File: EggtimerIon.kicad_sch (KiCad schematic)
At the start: 33 parts, among them J1 Conn_01x02, J2 Conn_01x03, J3 B2B-PH-K-S, Q1 IRLML6244, Q2 IRLML6244, U1 ESP32-WROOM-32-N4, U2 MPU-6050, U3 MS5611-01BA, U5 AP2112K-3.3

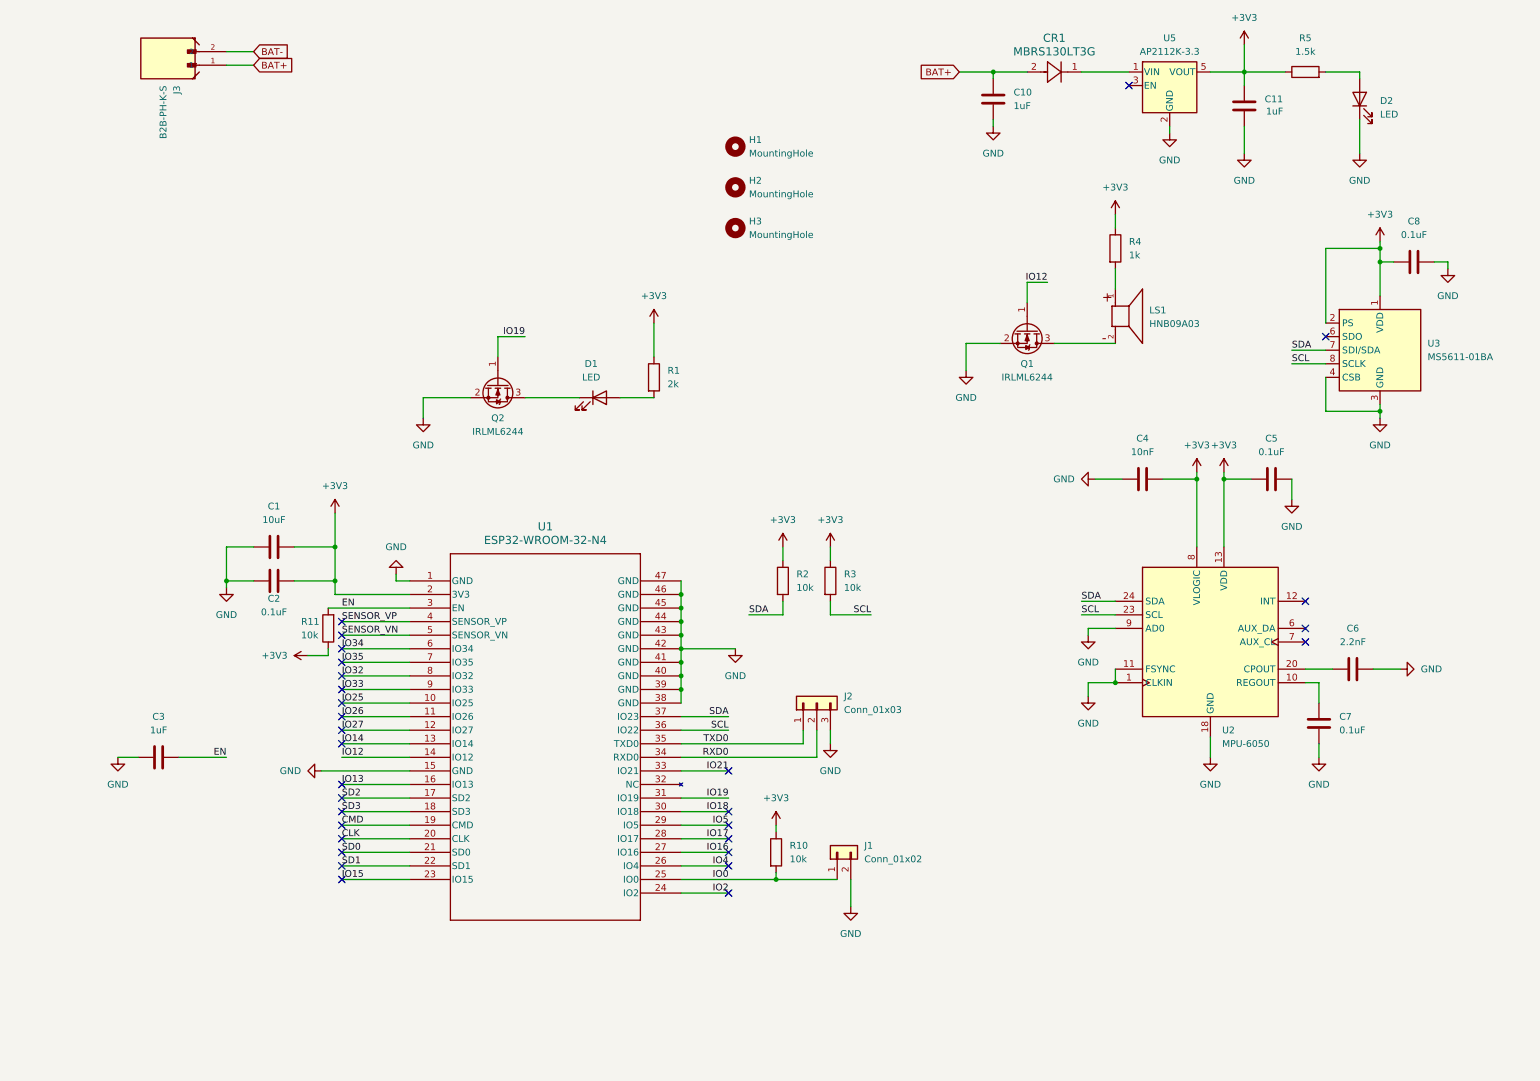
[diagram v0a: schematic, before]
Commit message: work
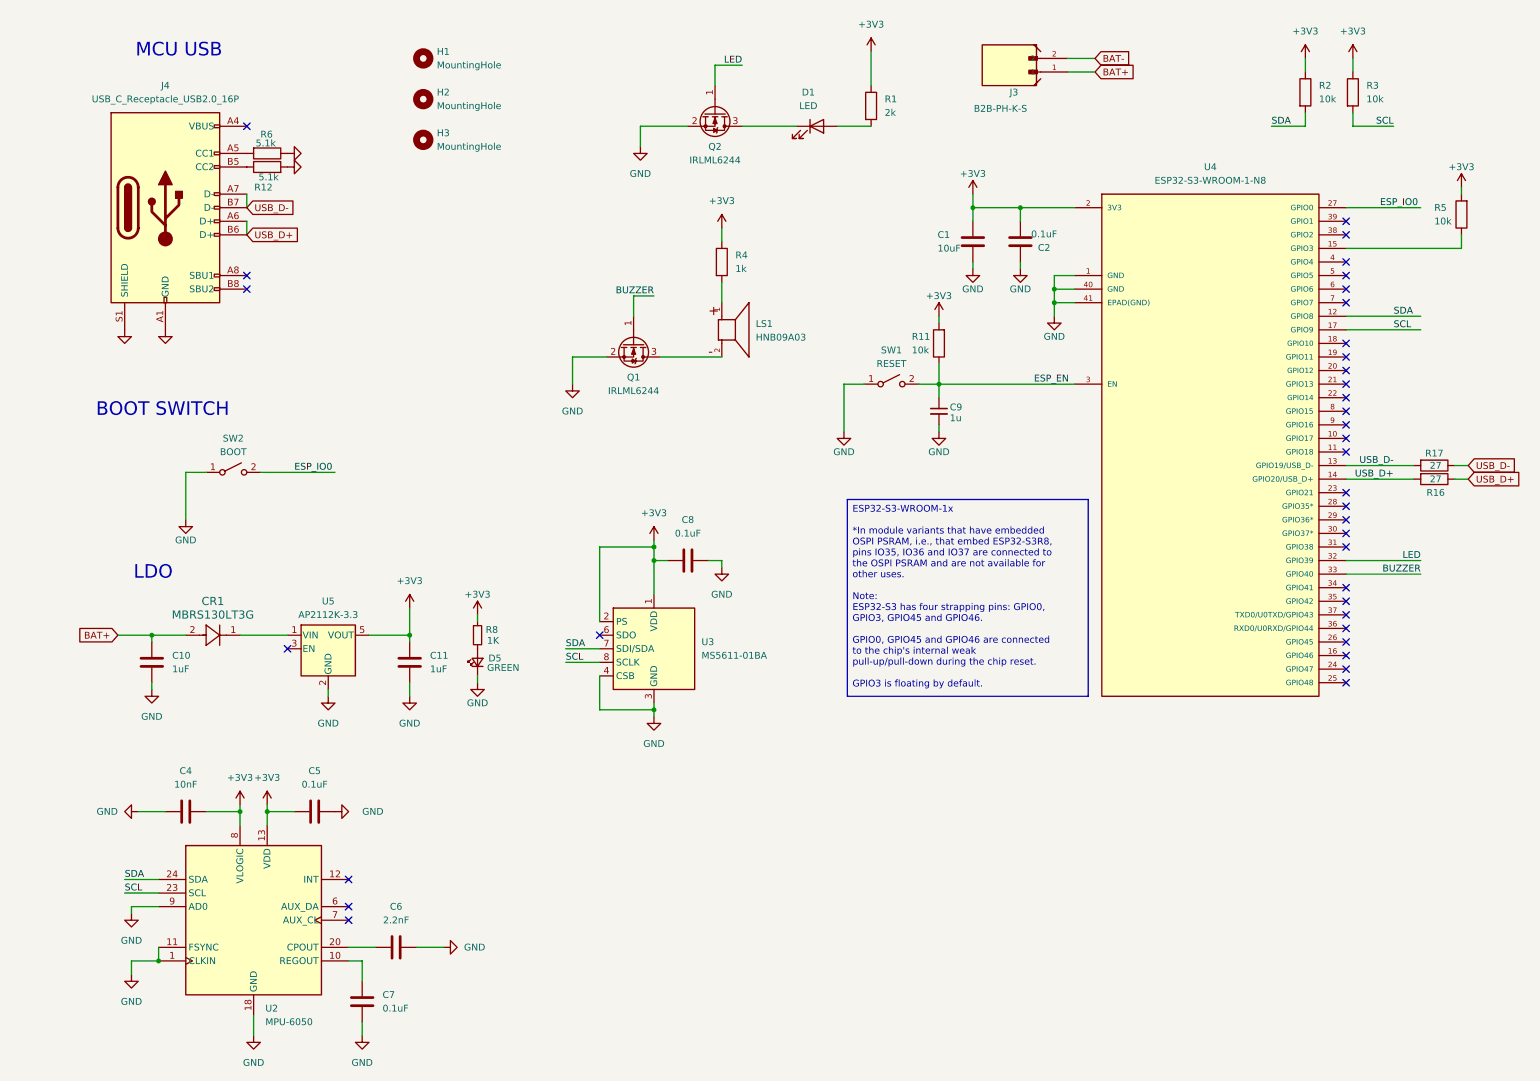
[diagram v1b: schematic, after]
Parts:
- removed C3: 1uF, Capacitor_SMD:C_0402_1005Metric, symbol Device:C
- removed D2: LED, LED_SMD:LED_0603_1608Metric, symbol Device:LED
- removed J1: Conn_01x02, Connector_PinHeader_2.54mm:PinHeader_1x02_P2.54mm_Vertical, symbol Connector_Generic:Conn_01x02
- removed J2: Conn_01x03, Connector_PinHeader_2.54mm:PinHeader_1x03_P2.54mm_Vertical, symbol Connector_Generic:Conn_01x03
- removed R10: 10k, Capacitor_SMD:C_0402_1005Metric, symbol Device:R
- removed U1: ESP32-WROOM-32-N4, RF_Module:ESP32-WROOM-32, symbol ESP32-WROOM-32-N4:ESP32-WROOM-32-N4
- added C9: 1u, Capacitor_SMD:C_0603_1608Metric, symbol Morten_Library.kicad_sym_9:C_Small
- added D5: GREEN, LED_SMD:LED_0603_1608Metric, symbol Morten_Library.kicad_sym_9:LED_Small
- added J4: USB_C_Receptacle_USB2.0_16P, Connector_USB:USB_C_Receptacle_Palconn_UTC16-G, symbol Connector:USB_C_Receptacle_USB2.0_16P
- added R12, R6: 5.1k, Resistor_SMD:R_0402_1005Metric, symbol Device:R
- added R16, R17: 27, Resistor_SMD:R_0402_1005Metric, symbol Device:R
- added R8: 1K, Resistor_SMD:R_0402_1005Metric, symbol Morten_Library.kicad_sym_9:R_Small
- added SW1: RESET, Button_Switch_SMD:SW_SPST_B3U-1000P, symbol Morten_Library.kicad_sym_9:SW_SPST
- added SW2: BOOT, Button_Switch_SMD:SW_SPST_B3U-1000P, symbol Morten_Library.kicad_sym_9:SW_SPST
- added U4: ESP32-S3-WROOM-1-N8, RF_Module:ESP32-S3-WROOM-1, symbol Morten_Library.kicad_sym_9:ESP32-S3-WROOM-1x-N8R8
- R5: value 1.5k -> 10k; LCSC C25867 -> C25744
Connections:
- net EN is gone; now on net +3V3: R11.2
- net +3V3: now also R5.2, R8.1, U4.2 (3V3); no longer R11.1, R5.1
- net GND: now also C9.2, D5.1 (K), J4.A1 (GND), J4.A12 (GND), J4.B1 (GND), J4.B12 (GND), J4.S1 (SHIELD), R12.2, R6.1, SW1.1 (A), SW2.1 (A), U4.1 (GND), U4.40 (GND), U4.41 (EPAD(GND))
- net SCL: now also U4.17 (GPIO9)
- net SDA: now also U4.12 (GPIO8)
- net IO12 renamed BUZZER
- net BUZZER: now also U4.33 (GPIO40)
- net IO19 renamed LED
- net LED: now also U4.32 (GPIO39)
- new net: J4.A4 (VBUS), J4.A9 (VBUS), J4.B4 (VBUS), J4.B9 (VBUS)
- new net: J4.A5 (CC1), R6.2
- new net: J4.B5 (CC2), R12.1
- new net: D5.2 (A), R8.2
- new net: R5.1, U4.15 (GPIO3)
- new net ESP_EN: C9.1, R11.1, SW1.2 (B), U4.3 (EN)
- new net ESP_IO0: SW2.2 (B), U4.27 (GPIO0)
- new net USB_D+: J4.A6 (D+), J4.B6 (D+), R16.1, R16.2, U4.14 (GPIO20/USB_D+)
- new net USB_D-: J4.A7 (D-), J4.B7 (D-), R17.1, R17.2, U4.13 (GPIO19/USB_D-)
- no-connect marks 30 -> 36
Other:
- note added: "BOOT SWITCH"
- note added: "LDO"
- note added: "MCU USB"
- moved on the sheet: C1, C10, C11, C2, C4, C5, C6, C7, C8, CR1, D1, H1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

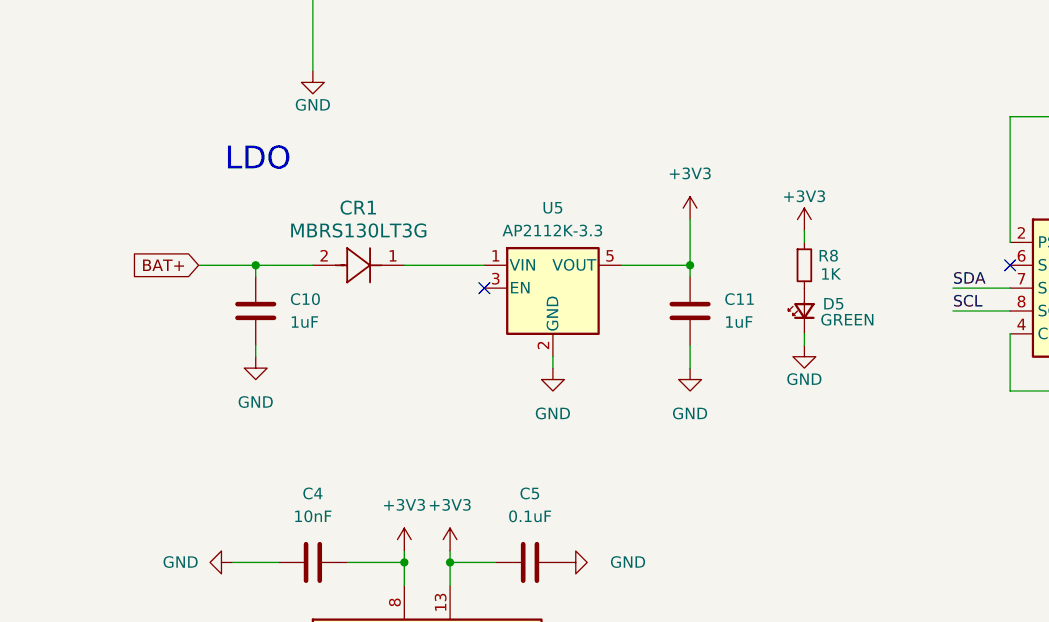
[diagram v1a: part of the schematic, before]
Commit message: Updates
work towards S3 module
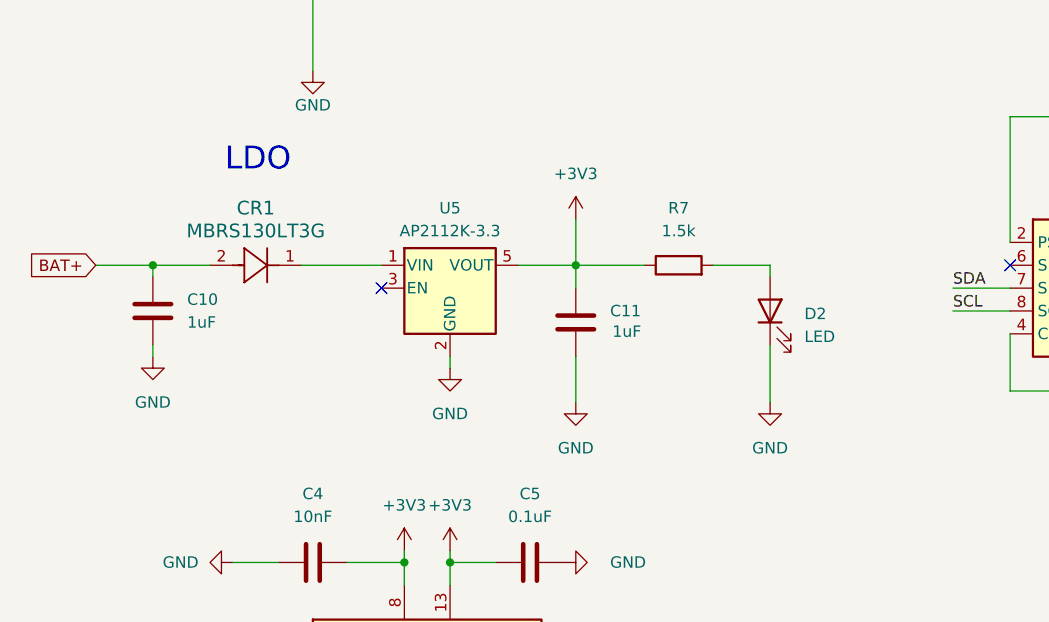
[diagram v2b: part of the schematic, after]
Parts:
- removed D5: GREEN, LED_SMD:LED_0603_1608Metric, symbol Morten_Library.kicad_sym_9:LED_Small
- removed R8: 1K, Resistor_SMD:R_0402_1005Metric, symbol Morten_Library.kicad_sym_9:R_Small
- added D2: LED, LED_SMD:LED_0603_1608Metric, symbol Device:LED
- added R7: 1.5k, Capacitor_SMD:C_0402_1005Metric, symbol Device:R
- CR1: footprint MBRS130L3TG:DIODE_SMB_2L_ONS -> Diode:DIODE_SMB_2L_ONS
- U5: footprint Package_TO_SOT_SMD:SOT-23-5 -> LDO:SOT_RG1_DIO
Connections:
- net +3V3: now also R7.1
- net GND: now also D2.1 (K)
- new net: D2.2 (A), R7.2
